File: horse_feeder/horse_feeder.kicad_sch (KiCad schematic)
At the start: 100 parts, among them J1 PWR, J10 Btn_RST, J11 Btn_USR2, J2 Moteur 2, J3 Moteur 1, J4 Proxi 1, J5 UART, J6 Proxi 2, J7 I2C, J8 PROG, J9 Btn_USR1, M1 SIM800L, Q1 Si7155DP, Q2 BUK766R060E, Q3 BUK766R060E, Q4 VP3203, Q5 VP3203, Q6 2N7002, U1 MCP16301x-xCH, U2 MIC4427, U3 ATmega644PA-P, U4 RTC, Y1 16MHz

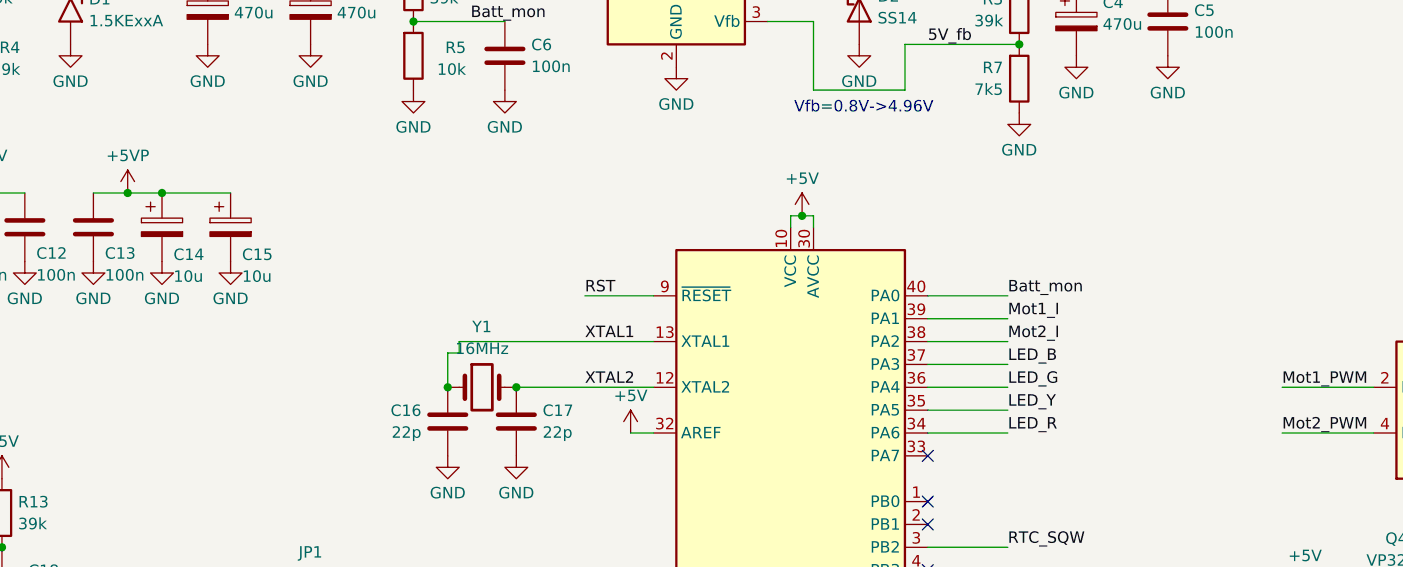
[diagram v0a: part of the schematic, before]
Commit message: a
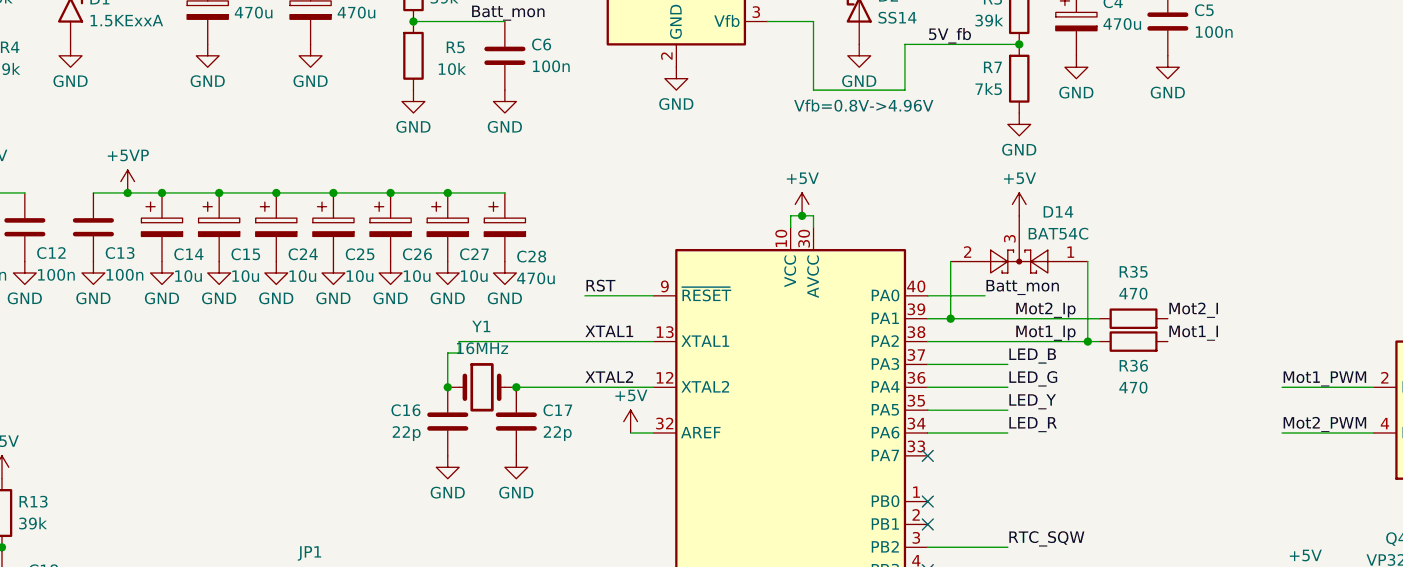
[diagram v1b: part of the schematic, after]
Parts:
- added C24, C25, C26, C27: 10u, Capacitor_SMD:C_0805_2012Metric_Pad1.18x1.45mm_HandSolder, symbol Device:C_Polarized
- added C28: 470u, Capacitor_THT:CP_Radial_D12.5mm_P5.00mm, symbol Device:C_Polarized
- added D14: BAT54C, Package_TO_SOT_SMD:SOT-23, symbol Diode:BAT54C
- added R35, R36: 470, Resistor_SMD:R_0805_2012Metric_Pad1.20x1.40mm_HandSolder, symbol Device:R
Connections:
- net +5V: now also D14.3
- net +5VP: now also C24.1, C25.1, C26.1, C27.1, C28.1
- net GND: now also C24.2, C25.2, C26.2, C27.2, C28.2
- net Mot1_I: now also R36.2; no longer U3.39 (PA1)
- net Mot2_I: now also R35.2; no longer U3.38 (PA2)
- new net Mot1_Ip: D14.1, R36.1, U3.38 (PA2)
- new net Mot2_Ip: D14.2, R35.1, U3.39 (PA1)
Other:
- moved on the sheet: C15
